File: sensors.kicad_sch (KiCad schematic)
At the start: 13 parts

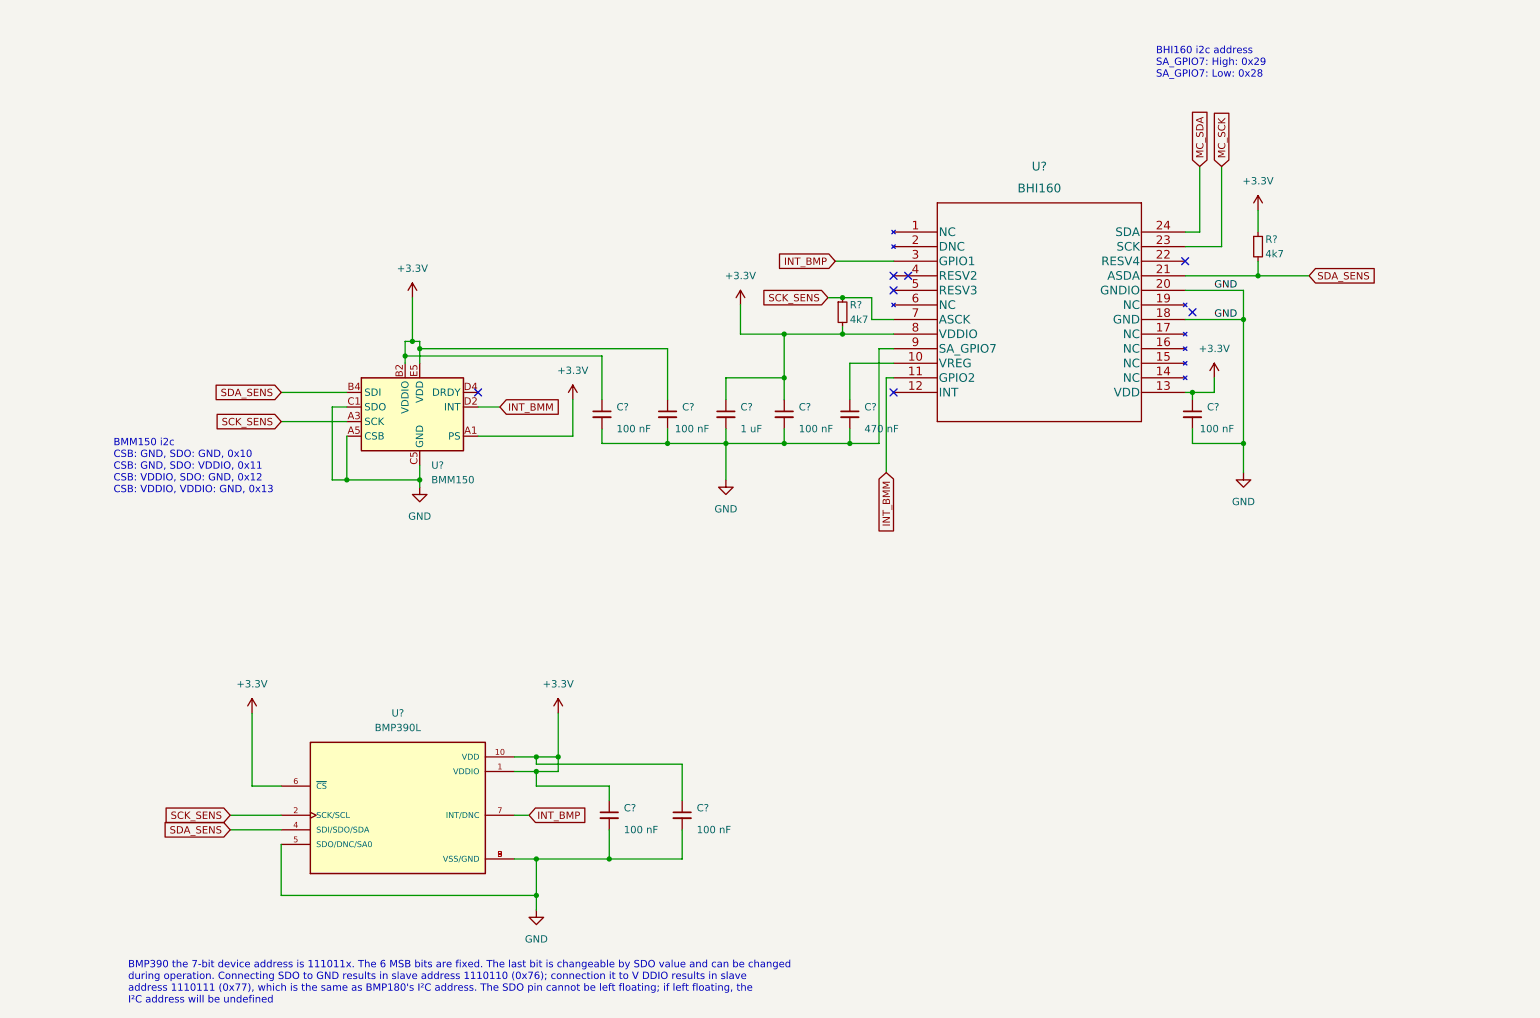
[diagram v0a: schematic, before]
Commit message: production version (2023)
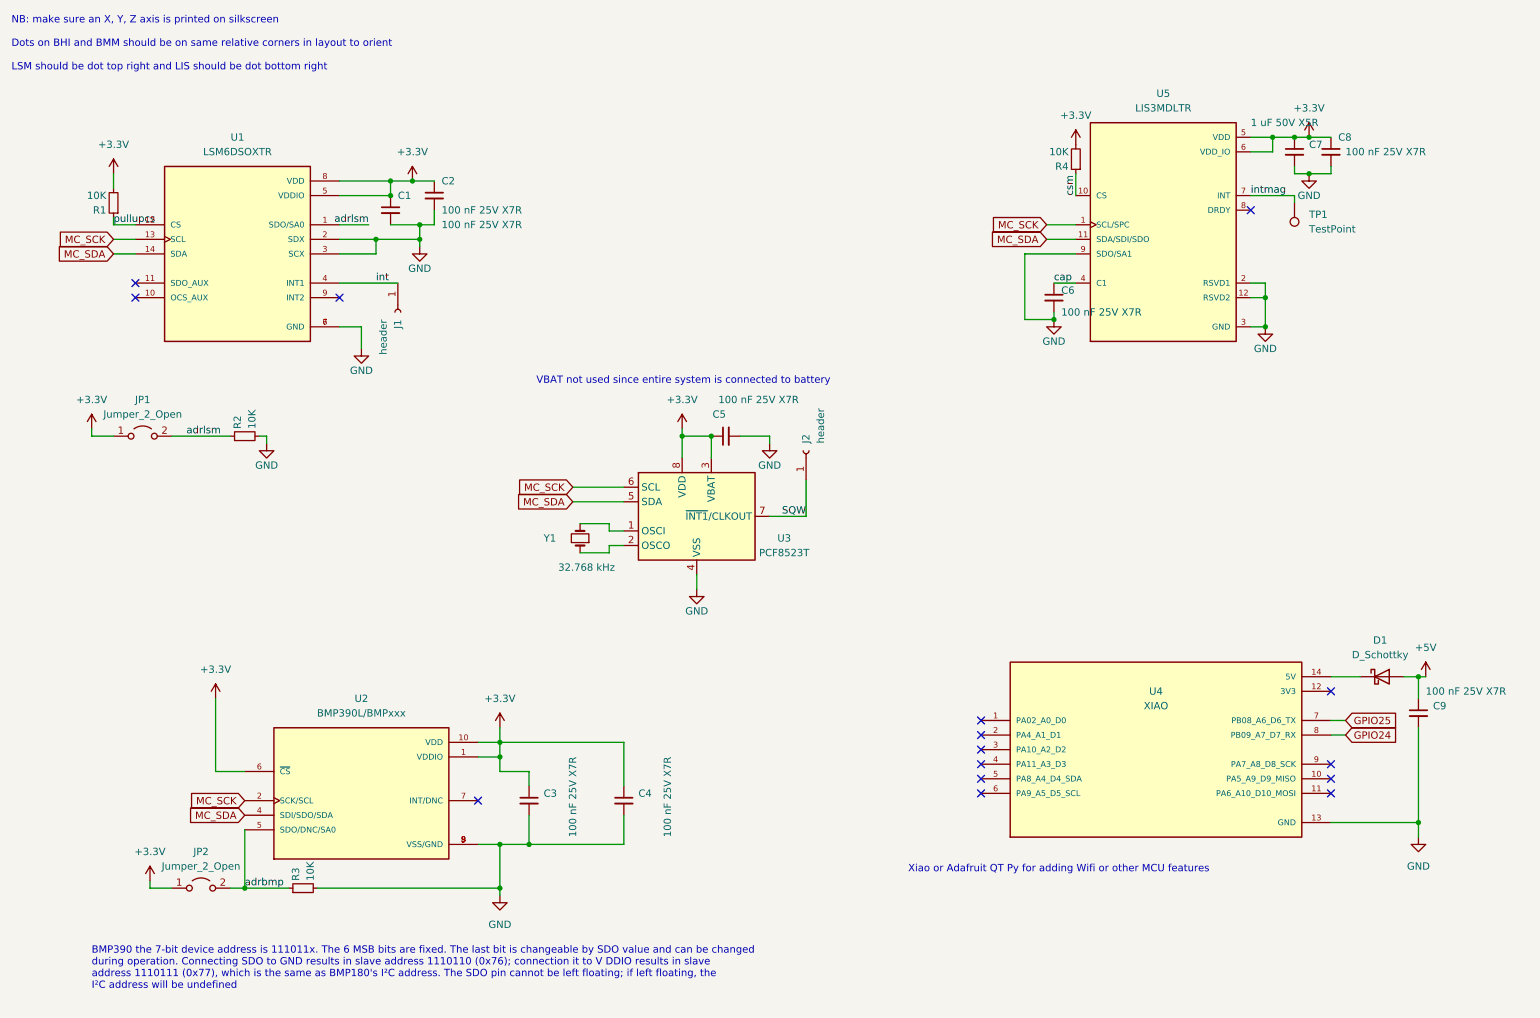
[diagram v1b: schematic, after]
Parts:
- removed C?: 470 nF, symbol Device:C_Small
- removed C? (x4): 100 nF, symbol Device:C_Small
- removed C?: 1 uF, symbol Device:C_Small
- removed R? (x2): 4k7, symbol Device:R_Small
- removed U?: BMM150, Package_CSP:WLCSP-12_1.56x1.56mm_P0.4mm, symbol Sensor_Magnetic:BMM150
- removed U?: BHI160, BHI160:BHI160, symbol BHI160:BHI160
- added C1, C2, C5, C6, C8, C9: 100 nF 25V X7R, Capacitor_SMD:C_0402_1005Metric, symbol Device:C_Small
- added C7: 1 uF 50V X5R, Capacitor_SMD:C_0603_1608Metric, symbol Device:C_Small
- added D1: D_Schottky, Diode_SMD:D_SMA, symbol Device:D_Schottky
- added J1, J2: header, Connector_PinHeader_2.54mm:PinHeader_1x01_P2.54mm_Vertical, symbol Connector:Conn_01x01_Female
- added JP1, JP2: Jumper_2_Open, Jumper:SolderJumper-2_P1.3mm_Open_RoundedPad1.0x1.5mm, symbol Jumper:Jumper_2_Open
- added R1, R2, R3, R4: 10K, Capacitor_SMD:C_0402_1005Metric_Pad0.74x0.62mm_HandSolder, symbol Device:R_Small
- added TP1: TestPoint, TestPoint:TestPoint_Pad_D1.0mm, symbol Connector:TestPoint
- added U1: LSM6DSOXTR, PowerIC:PQFN50P250X300X86-14N, symbol lsm6dso:LSM6DSOXTR
- added U3: PCF8523T, Package_SO:SOIC-8_3.9x4.9mm_P1.27mm, symbol Timer_RTC:PCF8523T
- added U4: XIAO, PowerIC:xiao, symbol xiao:102010388
- added U5: LIS3MDLTR, PowerIC:LIS3MDLTR, symbol lis3mdl:LIS3MDLTR
- added Y1: 32.768 kHz, Crystal:Crystal_SMD_3215-2Pin_3.2x1.5mm, symbol Device:Crystal_Small
- C3, C4: renamed from C?; value 100 nF -> 100 nF 25V X7R; footprint (none) -> Capacitor_SMD:C_0402_1005Metric; JCLPCB (none) -> C307331; Vendor (none) -> C307331
- U2: renamed from U?; value BMP390L -> BMP390L/BMPxxx; footprint XDCR_BMP390L -> PowerIC:XDCR_BMP390L; JCLPCB (none) -> C779278; Vendor (none) -> C779278
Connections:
- net SCK_SENS is gone; now on net MC_SCK: U2.2 (SCK/SCL)
- net SDA_SENS is gone; now on net MC_SDA: U2.4 (SDI/SDO/SDA)
- net +3V3: now also C1.1, C2.1, C5.1, C7.1, C8.1, JP1.1 (A), JP2.1 (A), R1.2, R4.2, U1.5 (VDDIO), U1.8 (VDD), U3.3 (VBAT), U3.8 (VDD), U5.5 (VDD), U5.6 (VDD_IO)
- net GND: now also C1.2, C2.2, C5.2, C6.2, C7.2, C8.2, C9.2, R2.2, R3.2, U1.2 (SDX), U1.3 (SCX), U1.6 (GND), U1.7 (GND), U3.4 (VSS), U4.13 (GND), U5.12 (RSVD2), U5.2 (RSVD1), U5.3 (GND), U5.9 (SDO/SA1); no longer U2.5 (SDO/DNC/SA0)
- net MC_SCK: now also U1.13 (SCL), U3.6 (SCL), U5.1 (SCL/SPC)
- net MC_SDA: now also U1.14 (SDA), U3.5 (SDA), U5.11 (SDA/SDI/SDO)
- net INT_BMP: no longer names the net of U2.7 (INT/DNC)
- new net: D1.1 (K), U4.14 (5V)
- new net: U3.1 (OSCI), Y1.2
- new net: U3.2 (OSCO), Y1.1
- new net +5V: C9.1, D1.2 (A)
- new net GPIO24: U4.8 (PB09_A7_D7_RX)
- new net GPIO25: U4.7 (PB08_A6_D6_TX)
- new net SQW: J2.1 (Pin_1), U3.7 (~{INT1}/CLKOUT)
- new net adrbmp: JP2.2 (B), R3.1, U2.5 (SDO/DNC/SA0)
- new net adrlsm: JP1.2 (B), R2.1, U1.1 (SDO/SA0)
- new net cap: C6.1, U5.4 (C1)
- new net csm: R4.1, U5.10 (CS)
- new net int: J1.1 (Pin_1), U1.4 (INT1)
- new net intmag: TP1.1, U5.7 (INT)
- new net pullupcs: R1.1, U1.12 (CS)
- no-connect marks 7 -> 15
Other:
- note added: "NB: make sure an X, Y, Z axis is printed on silkscreen Dots on BHI and BMM should be on same relative corners in layout to orient LSM should be dot top right and LIS should be dot bottom right"
- note added: "VBAT not used since entire system is connected to battery"
- note added: "Xiao or Adafruit QT Py for adding Wifi or other MCU features"
- note removed: "BHI160 i2c address SA_GPIO7: High: 0x29 SA_GPIO7: Low: 0x28"
- note removed: "BMM150 i2c CSB: GND, SDO: GND, 0x10 CSB: GND, SDO: VDDIO, 0x11 CSB: VDDIO, SDO: GND, 0x12 CSB: VDDIO, VDDIO: GND, 0x13"
- moved on the sheet: C3, C4, U2
